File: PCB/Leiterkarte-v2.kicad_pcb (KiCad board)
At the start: 4 copper layers, 70 x 70 mm, 59 parts

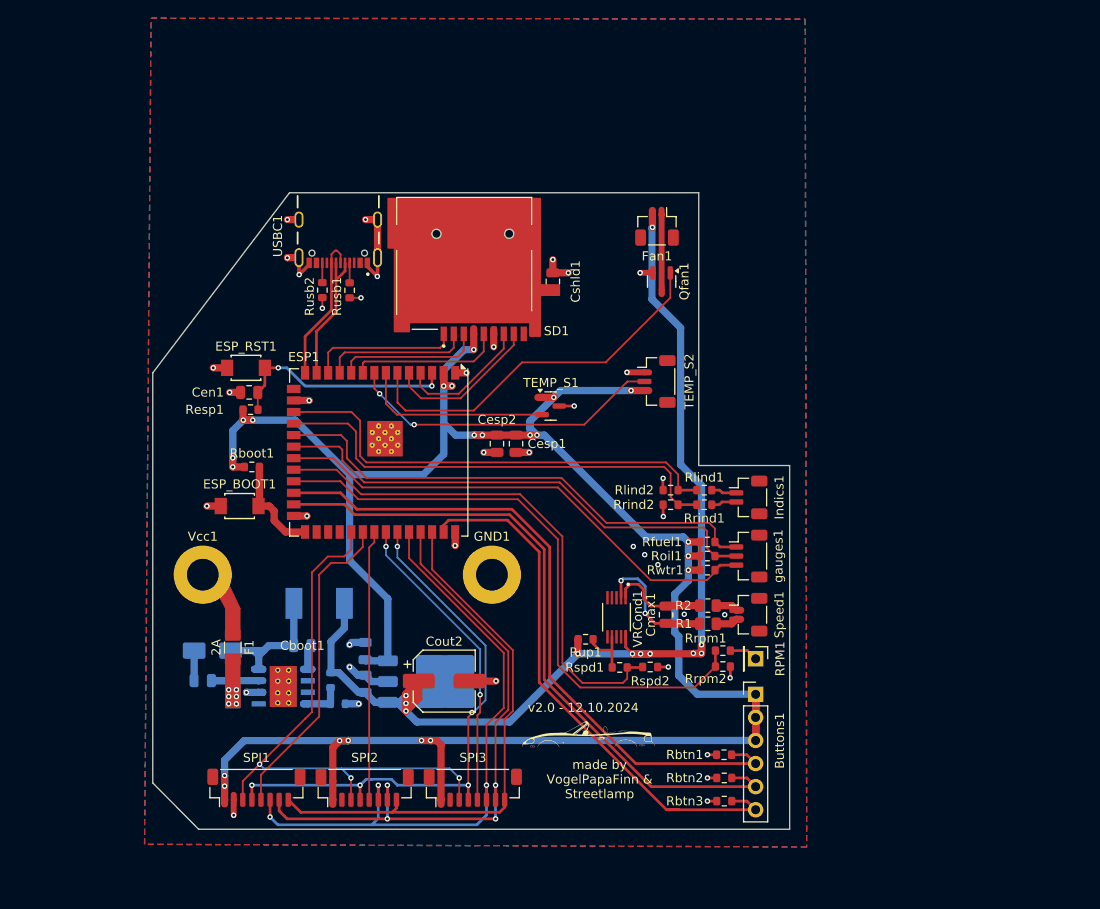
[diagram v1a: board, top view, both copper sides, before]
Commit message: PCB Version 2.1
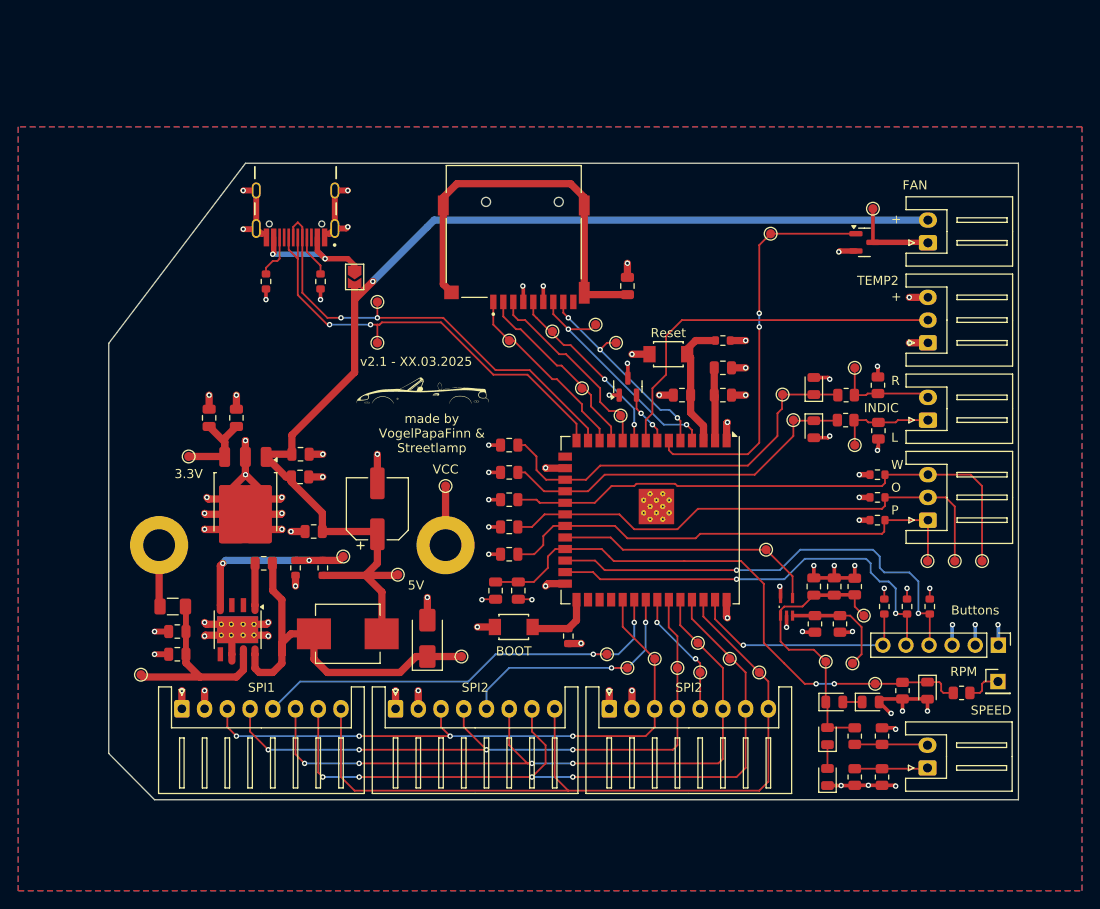
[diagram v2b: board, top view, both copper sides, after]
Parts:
- removed 3.3V1: LD39150DT33, Package_TO_SOT_SMD:TO-252-3_TabPin2
- removed Cmax1: 1nF, Capacitor_SMD:C_0805_2012Metric
- removed Rlind1, Rrind1, Rrpm1: 40k, Resistor_SMD:R_0603_1608Metric
- removed Rlind2, Rrind2, Rrpm2, Rspd1, Rup1: 10k, Resistor_SMD:R_0603_1608Metric
- removed Rspd2: 20k, Resistor_SMD:R_0603_1608Metric
- removed VRCond1: MAX9924UAUB_T, MAX9924UAUB:SOP50P490X110-10N
- added Cf1: spare, Capacitor_SMD:C_0805_2012Metric, F.Cu at (157.5, 91.5)
- added Cf10: C, Capacitor_SMD:C_0805_2012Metric, F.Cu at (124.0, 85.0)
- added Cf12: C, Capacitor_SMD:C_0805_2012Metric, F.Cu at (124.0, 88.0)
- added Cf13: C, Capacitor_SMD:C_0805_2012Metric, F.Cu at (124.0, 76.0)
- added Cf16: C, Capacitor_SMD:C_0805_2012Metric, F.Cu at (124.0, 79.0)
- added Cf3: spare, Capacitor_SMD:C_0805_2012Metric, F.Cu at (159.8, 91.5)
- added Cf5: C, Capacitor_SMD:C_0805_2012Metric, F.Cu at (125.0, 92.0)
- added Cf6: C, Capacitor_SMD:C_0805_2012Metric, F.Cu at (122.5, 92.0)
- added Cf8: C, Capacitor_SMD:C_0805_2012Metric, F.Cu at (124.0, 82.0)
- added Cin1.1: C, Capacitor_SMD:C_0805_2012Metric, F.Cu at (87.5, 99.0)
- added Cin2.1: C, Capacitor_SMD:C_0805_2012Metric, F.Cu at (101.0, 79.5)
- added Cout1.1: C, Capacitor_SMD:C_0805_2012Metric, F.Cu at (91.0, 73.0)
- added Cout2.1: C, Capacitor_SMD:C_0805_2012Metric, F.Cu at (102.5, 85.5)
- added D2: D_Schottky, Diode_SMD:D_0805_2012Metric, F.Cu at (159.8, 104.2)
- added D3: D_Schottky, Diode_SMD:D_0805_2012Metric, F.Cu at (159.0, 112.5)
- added D4: D_Schottky, Diode_SMD:D_0805_2012Metric, F.Cu at (159.0, 108.0)
- added D5: D_Zener 3.3V, Diode_SMD:D_0805_2012Metric, F.Cu at (170.0, 103.0)
- added D6: D_Schottky, Diode_SMD:D_0805_2012Metric, F.Cu at (163.8, 104.2)
- added D7: D_Zener 3.3V, Diode_SMD:D_0805_2012Metric, F.Cu at (157.5, 69.5)
- added D8: D_Zener 3.3V, Diode_SMD:D_0805_2012Metric, F.Cu at (157.5, 74.2)
- added JP1: SolderJumper_2_Open, Jumper:SolderJumper-2_P1.3mm_Open_TrianglePad1.0x1.5mm, F.Cu at (107.0, 57.5)
- added R10: 100k, Resistor_SMD:R_0805_2012Metric, F.Cu at (165.0, 112.5)
- added R11: 100k, Resistor_SMD:R_0805_2012Metric, F.Cu at (165.0, 108.0)
- added R12: spare, Resistor_SMD:R_0805_2012Metric, F.Cu at (162.0, 91.5)
- added R13: 10k, Resistor_SMD:R_0805_2012Metric, F.Cu at (167.2, 103.0)
- added R3: 100k, Resistor_SMD:R_0805_2012Metric, F.Cu at (157.6, 95.7)
- added R4: 10k, Resistor_SMD:R_0805_2012Metric, F.Cu at (160.4, 95.7)
- added R5: 10k, Resistor_SMD:R_0805_2012Metric, F.Cu at (173.8, 103.2)
- added R6: 10k, Resistor_SMD:R_0805_2012Metric, F.Cu at (161.0, 73.2)
- added R7: 10k, Resistor_SMD:R_0805_2012Metric, F.Cu at (161.1, 70.5)
- added R8: 40k, Resistor_SMD:R_0805_2012Metric, F.Cu at (164.6, 69.4)
- added R9: 40k, Resistor_SMD:R_0805_2012Metric, F.Cu at (164.6, 74.4)
- added TP1: TestPoint_Small, TestPoint:TestPoint_Pad_D1.0mm, F.Cu at (83.5, 101.2)
- added TP10: TestPoint_Small, TestPoint:TestPoint_Pad_D1.0mm, F.Cu at (162.0, 76.0)
- added TP11: TestPoint_Small, TestPoint:TestPoint_Pad_D1.0mm, F.Cu at (162.0, 67.5)
- added TP12: TestPoint_Small, TestPoint:TestPoint_Pad_D1.0mm, F.Cu at (164.2, 102.2)
- added TP13: TestPoint_Small, TestPoint:TestPoint_Pad_D1.0mm, F.Cu at (109.5, 60.2)
- added TP14: TestPoint_Small, TestPoint:TestPoint_Pad_D1.0mm, F.Cu at (109.5, 64.8)
- added TP15: TestPoint_Small, TestPoint:TestPoint_Pad_D1.0mm, F.Cu at (140.0, 99.5)
- added TP16: TestPoint_Small, TestPoint:TestPoint_Pad_D1.0mm, F.Cu at (142.5, 100.5)
- added TP18: TestPoint_Small, TestPoint:TestPoint_Pad_D1.0mm, F.Cu at (144.8, 97.8)
- added TP19: TestPoint_Small, TestPoint:TestPoint_Pad_D1.0mm, F.Cu at (148.2, 99.5)
- added TP20: TestPoint_Small, TestPoint:TestPoint_Pad_D1.0mm, F.Cu at (151.5, 101.0)
- added TP21: TestPoint_Small, TestPoint:TestPoint_Pad_D1.0mm, F.Cu at (145.0, 101.0)
- added TP22: TestPoint_Small, TestPoint:TestPoint_Pad_D1.0mm, F.Cu at (137.0, 100.5)
- added TP23: TestPoint_Small, TestPoint:TestPoint_Pad_D1.0mm, F.Cu at (134.8, 99.0)
- added TP24: TestPoint_Small, TestPoint:TestPoint_Pad_D1.0mm, F.Cu at (128.8, 63.5)
- added TP25: TestPoint_Small, TestPoint:TestPoint_Pad_D1.0mm, F.Cu at (136.2, 72.8)
- added TP26: TestPoint_Small, TestPoint:TestPoint_Pad_D1.0mm, F.Cu at (133.5, 62.8)
- added TP27: TestPoint_Small, TestPoint:TestPoint_Pad_D1.0mm, F.Cu at (135.8, 64.8)
- added TP28: TestPoint_Small, TestPoint:TestPoint_Pad_D1.0mm, F.Cu at (124.0, 64.5)
- added TP29: TestPoint_Small, TestPoint:TestPoint_Pad_D1.0mm, F.Cu at (132.0, 69.8)
- added TP3: TestPoint_Small, TestPoint:TestPoint_Pad_D1.0mm, F.Cu at (118.8, 99.2)
- added TP30: TestPoint_Small, TestPoint:TestPoint_Pad_D1.0mm, F.Cu at (155.2, 73.2)
- added TP31: TestPoint_Small, TestPoint:TestPoint_Pad_D1.0mm, F.Cu at (154.1, 70.4)
- added TP32: TestPoint_Small, TestPoint:TestPoint_Pad_D1.0mm, F.Cu at (158.8, 99.8)
- added TP33: TestPoint_Small, TestPoint:TestPoint_Pad_D1.0mm, F.Cu at (117.0, 80.5)
- added TP34: TestPoint_Small, TestPoint:TestPoint_Pad_D1.0mm, F.Cu at (163.0, 94.8)
- added TP35: TestPoint_Small, TestPoint:TestPoint_Pad_D1.0mm, F.Cu at (161.8, 100.0)
- added TP36: TestPoint_Small, TestPoint:TestPoint_Pad_D1.0mm, F.Cu at (152.2, 87.5)
- added TP37: TestPoint_Small, TestPoint:TestPoint_Pad_D1.0mm, F.Cu at (152.8, 52.8)
- added TP38: TestPoint_Small, TestPoint:TestPoint_Pad_D1.0mm, F.Cu at (164.0, 50.0)
- added TP39: TestPoint_Small, TestPoint:TestPoint_Pad_D1.0mm, F.Cu at (111.8, 90.2)
- added TP4: TestPoint_Small, TestPoint:TestPoint_Pad_D1.0mm, F.Cu at (105.8, 88.2)
- added TP5: TestPoint_Small, TestPoint:TestPoint_Pad_D1.0mm, F.Cu at (88.8, 77.2)
- added TP7: TestPoint_Small, TestPoint:TestPoint_Pad_D1.0mm, F.Cu at (170.0, 88.8)
- added TP8: TestPoint_Small, TestPoint:TestPoint_Pad_D1.0mm, F.Cu at (173.0, 88.8)
- added TP9: TestPoint_Small, TestPoint:TestPoint_Pad_D1.0mm, F.Cu at (176.0, 88.8)
- added U1: LMV321, LMV321SEG-7:SOT65P210X110-5N, F.Cu at (154.5, 93.8)
- added V3.31: LD39150DT33, Package_TO_SOT_SMD:TO-252-3_TabPin2, F.Cu at (95.0, 82.3)
- 5V1, Cboot1, Cin1, Cin2, Cout1, D1, L1, Rfbb1, Rfbt1: moved to F.Cu
- Fan1, Indics1, Speed1: footprint Connector_JST:JST_SH_BM02B-SRSS-TB_1x02-1MP_P1.00mm_Vertical -> Connector_JST:JST_XH_S2B-XH-A_1x02_P2.50mm_Horizontal
- R1, R2: value 10k -> 40k
- Rfuel1, Roil1: value 100 -> 240
- Rwtr1: value 100 -> 3k
- SPI1, SPI2, SPI3: footprint Connector_JST:JST_SH_BM08B-SRSS-TB_1x08-1MP_P1.00mm_Vertical -> Connector_JST:JST_XH_S8B-XH-A_1x08_P2.50mm_Horizontal
- TEMP_S1: value MCP9700Ax-ETT -> Conn_01x03_Pin; footprint Package_TO_SOT_SMD:SOT-23 -> Connector_JST:JST_XH_S3B-XH-A_1x03_P2.50mm_Horizontal
- TEMP_S2: value Conn_01x03_Pin -> MCP9700Ax-ETT; footprint Connector_JST:JST_SH_BM03B-SRSS-TB_1x03-1MP_P1.00mm_Vertical -> Package_TO_SOT_SMD:SOT-23
- gauges1: footprint Connector_JST:JST_SH_BM03B-SRSS-TB_1x03-1MP_P1.00mm_Vertical -> Connector_JST:JST_XH_S3B-XH-A_1x03_P2.50mm_Horizontal
- moved Resp1 52.5 mm to (147.5, 64.5), turned to 180 degrees
- moved Cen1 47.6 mm to (143.0, 70.5)
- moved ESP_RST1 46.5 mm to (141.5, 66.0)
- moved TEMP_S1 42.1 mm to (170.1, 64.8), turned to 90 degrees
- moved G*** 42.0 mm to (114.5, 69.5)
- moved Rboot1 39.5 mm to (130.5, 97.0), turned to -90 degrees
- moved ESP_BOOT1 33.0 mm to (124.5, 96.0)
- moved ESP1 30.8 mm to (139.5, 84.2)
- moved Fan1 29.9 mm to (170.1, 53.8), turned to 90 degrees
- moved Rbtn3 29.4 mm to (167.8, 93.8), turned to 90 degrees
- moved Cout1 29.3 mm to (94.0, 73.0)
- moved Rbtn1 27.9 mm to (170.2, 93.8), turned to 90 degrees
- moved Buttons1 27.2 mm to (177.8, 98.0), turned to -90 degrees
- moved RPM1 26.8 mm to (177.8, 102.0), turned to 0 degrees
- moved Cin2 26.2 mm to (101.0, 77.0), turned to 0 degrees
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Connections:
- ESP1 pad 17: LIndicator -> RIndicator
- ESP1 pad 18: RIndicator -> LIndicator
- ESP1 pad 19: Fuel -> WTemp
- ESP1 pad 21: WTemp -> Fuel
- R2 pad 2: Net-(VRCond1-IN+) -> GND
- Rbtn2 pad 1: Button2 -> GND
- Rbtn2 pad 2: GND -> Button3
- Rbtn3 pad 1: GND -> Button2
- Rbtn3 pad 2: Button3 -> GND
- TEMP_S1 pad 1: +3.3V -> GND
- TEMP_S1 pad 2: TEMP1 -> TEMP2
- TEMP_S1 pad 3: GND -> +3.3V
- TEMP_S2 pad 1: GND -> +3.3V
- TEMP_S2 pad 2: TEMP2 -> TEMP1
- TEMP_S2 pad 3: +3.3V -> GND
- USBC1 pad A4_B9: unconnected-(USBC1-VBUS-PadA4_B9) -> Net-(JP1-A)
- USBC1 pad B4_A9: unconnected-(USBC1-VBUS__1-PadB4_A9) -> Net-(JP1-A)
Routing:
- net +3.3V: track 263.5 -> 47.0 mm, vias 22 -> 16
- net GND: track 80.3 -> 164.5 mm, vias 40 -> 71
- net Net-(Cshld1-Pad2): track 0.00 -> 42.9 mm
- net Button3: track 61.1 -> 25.3 mm, vias 0 -> 1
- net USB_D-: track 15.8 -> 50.5 mm, vias 0 -> 2
- net USB_D+: track 17.0 -> 49.7 mm, vias 0 -> 2
- net Speed: track 57.7 -> 29.2 mm
- net Button2: track 75.1 -> 47.0 mm, vias 0 -> 2
- net BL: track 60.5 -> 88.1 mm
- net Net-(5V1-PH): track 15.9 -> 43.0 mm
- net Button1: track 74.6 -> 50.6 mm, vias 0 -> 2
- net CS3: track 33.9 -> 14.1 mm
- net Net-(D2-K): track 14.4 -> 31.2 mm, vias 2 -> 0
- net RST: track 68.4 -> 84.3 mm
- net Net-(5V1-VSENSE): track 4.71 -> 20.4 mm, vias 0 -> 2
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- added copper zone on B.Cu, net +3.3V
- added copper zone on F.Cu, net +3.3V
- removed copper zone on B.Cu, net GND
- removed copper zone on F.Cu, net GND
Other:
- board size 70 x 70 mm -> 100 x 70 mm
- board text added: "+"
- board text added: "3.3V"
- board text added: "5V"
- board text added: "BOOT"
- board text added: "Buttons"
- board text added: "FAN"
- board text added: "INDIC"
- board text added: "L"
- board text added: "O"
- board text added: "P"
- board text added: "R"
- board text added: "RPM"
- board text added: "Reset"
- board text added: "SPEED"
- board text added: "SPI1"
- board text added: "SPI2"
- board text added: "TEMP2"
- board text added: "VCC"
- board text added: "W"
- board text added: "v2.1 - XX.03.2025"
- board text removed: "+-"
- board text removed: "-+"
- board text removed: "-O+"
- board text removed: "FOW"
- board text removed: "LR"
- board text removed: "v2.0 - 12.10.2024"
